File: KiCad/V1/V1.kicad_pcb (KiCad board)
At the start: 4 copper layers, 130.8 x 93.1 mm, 84 parts, among them Q1 Q_NMOS_GSD, Q2 Q_NMOS_GSD, U1 LMG1210RVRR, U2 OPA2677IDDA, U3 OPA2677IDDA, U4 OPA859QDSGRQ1, U5 OPA859QDSGRQ1, U6 OPA859QDSGRQ1

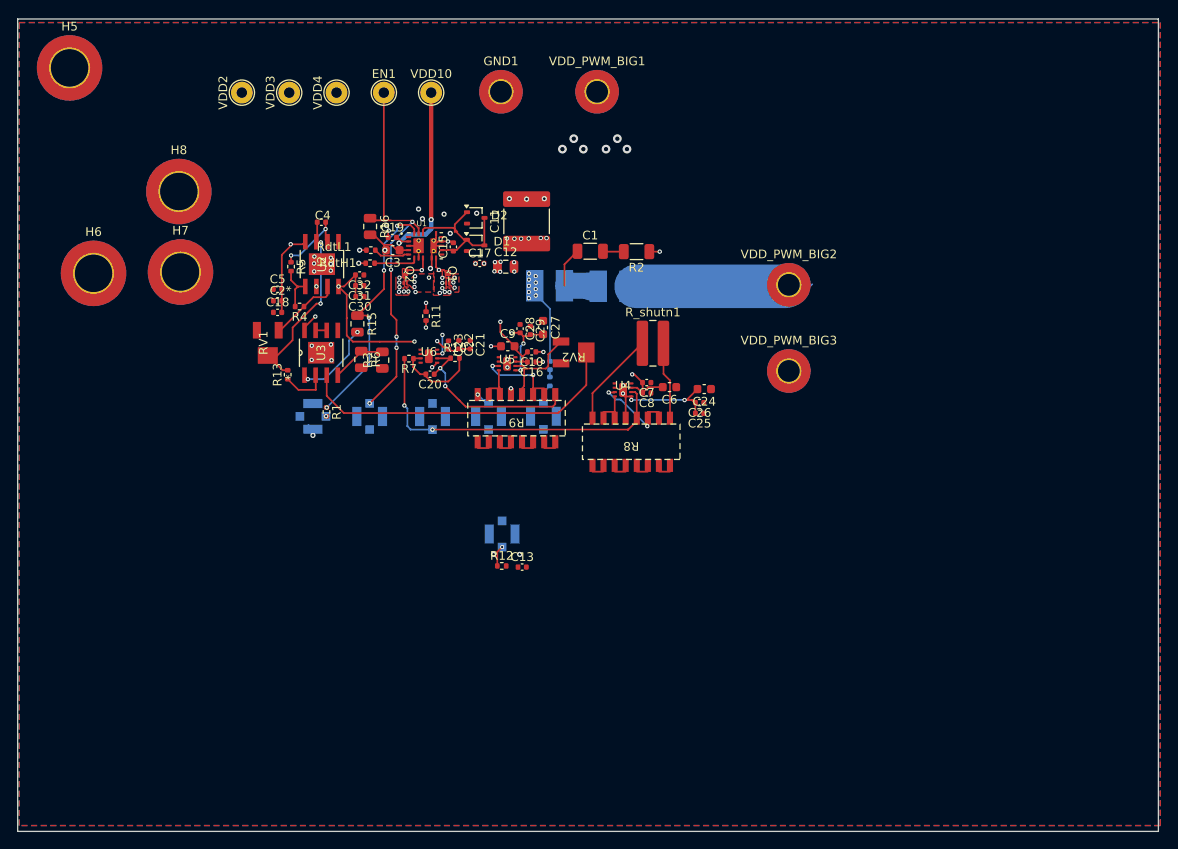
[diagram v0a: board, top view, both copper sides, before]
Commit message: V1 done
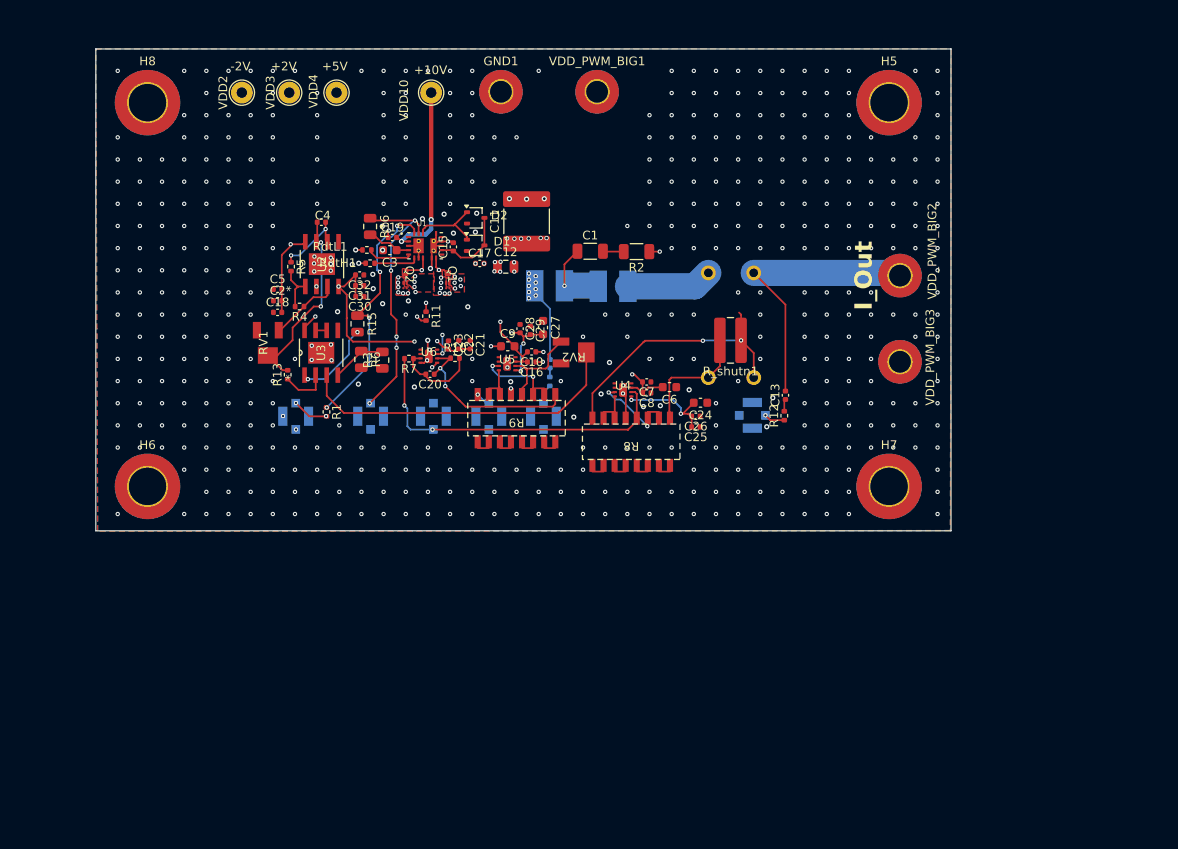
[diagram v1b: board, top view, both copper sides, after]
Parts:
- removed EN1: MountingHole_Pad, TestPoint:TestPoint_THTPad_D2.5mm_Drill1.2mm
- removed PWM_IN1, Pre_Filter2, Pre_Filter3, Pre_Filter4: Conn_Coaxial, Connector_Coaxial:U.FL_Molex_MCRF_73412-0110_Vertical
- added EN1_coax1: Conn_Coaxial, Connector_Coaxial:U.FL_Molex_MCRF_73412-0110_Vertical, B.Cu at (118.5, 61.5)
- added PWM_External1: Conn_Coaxial, Connector_Coaxial:U.FL_Molex_MCRF_73412-0110_Vertical, B.Cu at (109.9, 61.5)
- added Pre_FilterV_ref1: Conn_Coaxial, Connector_Coaxial:U.FL_Molex_MCRF_73412-0110_Vertical, B.Cu at (132.0, 61.5)
- added T1: Transformer_1P_1S, MyFootprints:MyTransformer, B.Cu at (159.8, 51.1)
- added V_duffsense1: Conn_Coaxial, Connector_Coaxial:U.FL_Molex_MCRF_73412-0110_Vertical, B.Cu at (125.7, 61.5)
- moved H5 94.0 mm to (177.9, 25.6)
- moved H7 84.9 mm to (177.9, 69.6)
- moved R12 36.7 mm to (165.9, 61.5), turned to 90 degrees
- moved C13 36.0 mm to (166.0, 59.1), turned to 90 degrees
- moved Post_Filter1 31.7 mm to (162.2, 61.4), turned to -90 degrees
- moved H6 25.2 mm to (92.9, 69.6)
- moved VDD_PWM_BIG2 12.8 mm to (179.1, 45.4)
- moved VDD_PWM_BIG3 12.8 mm to (179.1, 55.3)
- moved H8 10.8 mm to (92.9, 25.6)
- moved R_shutn1 8.90 mm to (159.7, 52.8), turned to 180 degrees
- moved C24 1.62 mm to (156.3, 60.0)
- moved C25 1.62 mm to (155.7, 62.8)
- moved C26 1.62 mm to (155.7, 61.5)
- moved RdtL1 0.45 mm to (118.0, 42.5)
- moved C3 0.34 mm to (120.7, 42.5)
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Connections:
- C13 pad 2: /OUT -> /+I_OUT
- Q1 pad 3: /VDD_PWM_Big -> /HS1
- Q1 pad 4: (no net) -> /VDD_PWM_Big
- Q1 pad 5: (no net) -> /HS1
- Q1 pad 6: (no net) -> /HS1
- Q2 pad 3: /HS1 -> GND
- Q2 pad 4: (no net) -> /HS1
- Q2 pad 5: (no net) -> GND
- Q2 pad 6: (no net) -> GND
- VDD_PWM_BIG3 pad 1: /-I_OUT -> GND
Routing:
- net /+I_OUT: track 0.00 -> 31.8 mm
- net Net-(T1-SA): track 10.2 -> 29.8 mm, vias 0 -> 2
- net /EN1: track 44.0 -> 30.6 mm
- net Net-(T1-AB): track 17.5 -> 9.86 mm
- net Net-(T1-SB): track 8.17 -> 13.1 mm
- net /PWM_External: track 0.08 -> 4.26 mm, vias 1 -> 2
- net Net-(C13-Pad1): track 0.00 -> 1.41 mm
- net GND: track 19.2 -> 20.3 mm, vias 53 -> 531
- net Net-(U1-PWM/LI): track 28.7 -> 29.7 mm
- net Net-(U1-DHL): track 4.12 -> 5.11 mm
- net /VDD10: track 21.8 -> 21.1 mm
- net Net-(C1-Pad1): track 7.22 -> 6.96 mm, vias 0 -> 1
- net /VDD_PWM_Big: vias 14 -> 16
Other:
- board size 130.8 x 93.1 mm -> 98 x 55.2 mm
- board text added: "+10V"
- board text added: "+2V"
- board text added: "+5V"
- board text added: "-2V"
- board text added: "I_Out"
